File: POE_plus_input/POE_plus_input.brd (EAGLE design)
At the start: 160 x 100 mm, 16 parts, among them U1 LM2673SX-5.0/NOPB

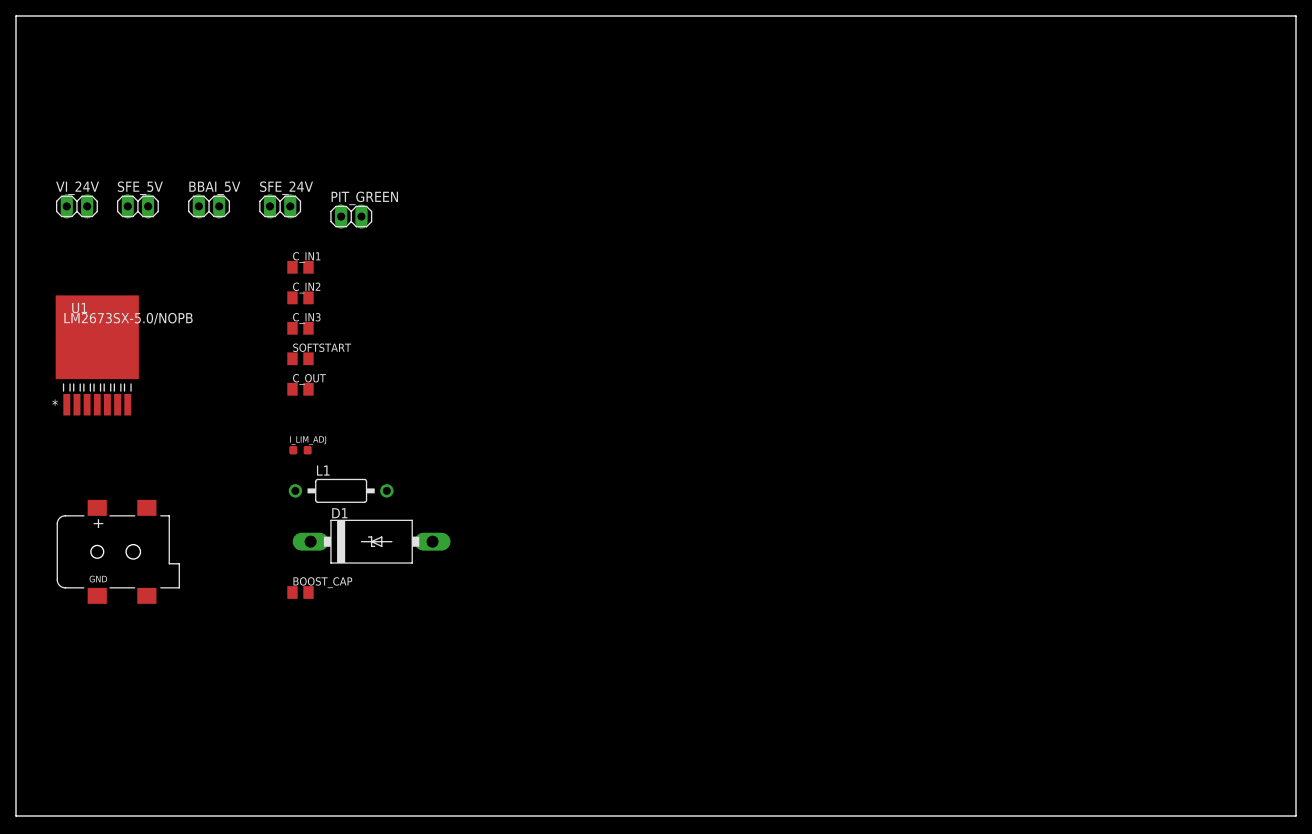
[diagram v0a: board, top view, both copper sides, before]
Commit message: POE, Vi board changes
POE Input Board: Added BB outline and mounting holes for BB-AI. Added small board standard outline and adjusted board size. Added attributes to regulator parts.
Valve Indicator: Added small board standard outline and adjusted board size.
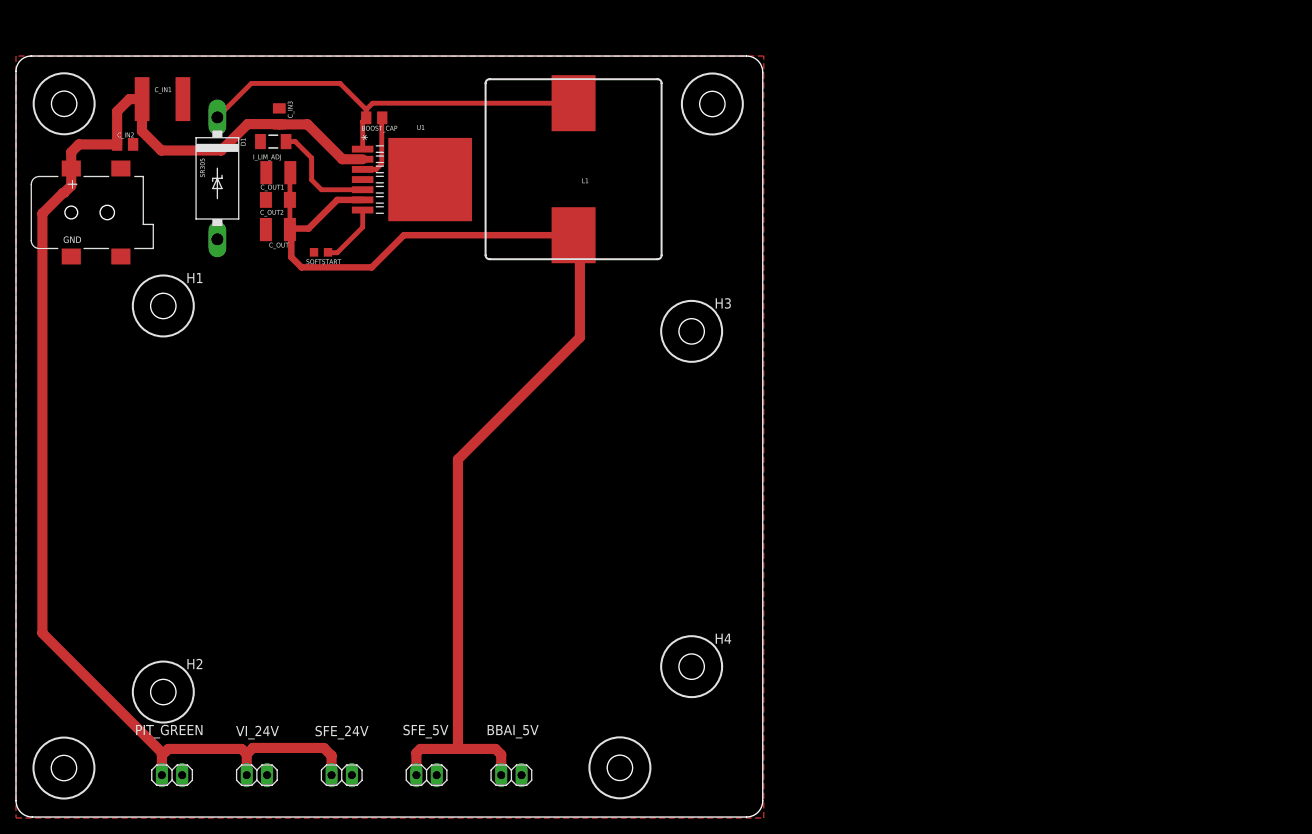
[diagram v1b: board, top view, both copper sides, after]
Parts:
- added C_OUT1: 100uF/16V, oresat-rcl:C1210K
- added C_OUT2: 33uF/16V, oresat-rcl:C1206K
- added H1, H2, H3, H4, H5, H6, H7, H8: #4-BARE_MOUNTING_HOLE/.300, mount:#4/.300-BARE+STD_NUT_OR_STAR_WASHER
- C_IN1: device oresat-rcl:C0805K -> oresat-rcl:C2220K
- C_OUT: value 180uF/16V -> 47uF/16V; device oresat-rcl:C0805K -> oresat-rcl:C1210K
- I_LIM_ADJ: device oresat-rcl:.0603-A-NOSILK -> oresat-rcl:1206-A
- L1: device rcl:IRF-1 -> oresat-rcl:22MMX22MMX12MM
- SOFTSTART: device oresat-rcl:C0805K -> oresat-rcl:C0603K
- moved BBAI_5V 80.5 mm to (61.9, 5.11)
- moved SFE_5V 79.7 mm to (51.3, 5.11)
- moved VI_24V 74.6 mm to (30.1, 5.11)
- moved PIT_GREEN 73.3 mm to (19.5, 5.11)
- moved SFE_24V 71.5 mm to (40.7, 5.11)
- moved BOOST_CAP 60.0 mm to (44.8, 87.3), turned to 180 degrees
- moved L1 49.6 mm to (69.7, 80.8), turned to 180 degrees
- moved D1 49.3 mm to (25.2, 79.7), turned to 270 degrees
- moved U1 46.0 mm to (51.6, 79.6), turned to 270 degrees
- moved POE_IN 42.5 mm to (6.91, 75.4)
- moved I_LIM_ADJ 38.7 mm to (32.2, 84.3)
- moved C_IN2 29.1 mm to (13.6, 83.9)
- moved C_IN1 27.2 mm to (18.3, 89.6)
- moved C_IN3 26.6 mm to (32.9, 87.5), turned to 90 degrees
- moved C_OUT 20.2 mm to (32.7, 73.3), turned to 180 degrees
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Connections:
- net +5V: now also C_OUT1.1, C_OUT2.1
- net GND: now also C_OUT1.2, C_OUT2.2
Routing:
- net +24V: track 0.00 -> 163.0 mm
- net +5V: track 0.00 -> 146.1 mm
- net N$2: track 0.00 -> 53.1 mm
- net N$6: track 0.00 -> 13.7 mm
- net N$7: track 0.00 -> 8.45 mm
- net N$1: track 0.00 -> 7.83 mm
- added copper zone on layer 1, net GND
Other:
- board size 160 x 100 mm -> 93.3 x 95.1 mm
